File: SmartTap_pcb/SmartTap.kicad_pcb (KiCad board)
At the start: 2 copper layers, 87.1 x 48.9 mm, 18 parts, among them U1 NT3H1101W0FTTJ

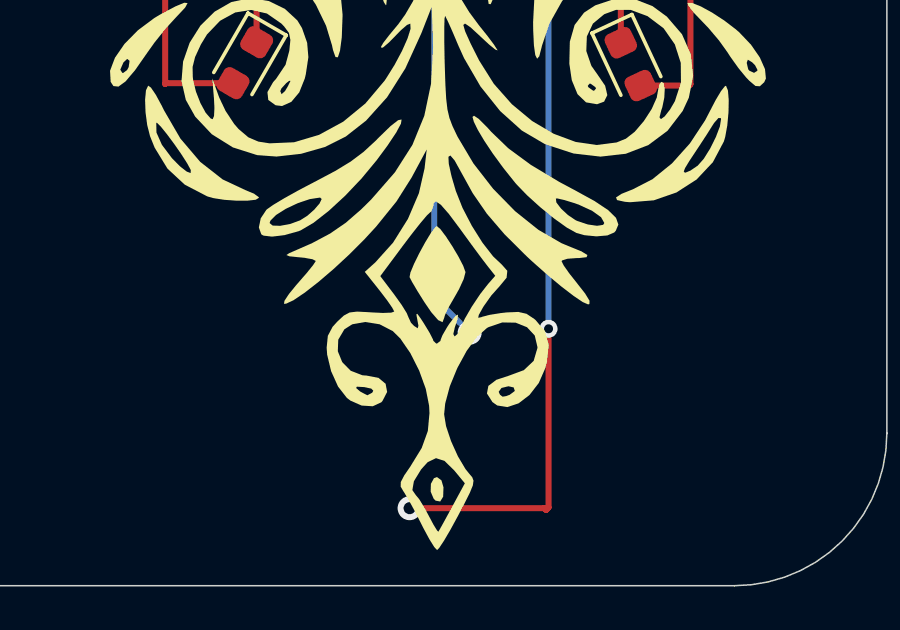
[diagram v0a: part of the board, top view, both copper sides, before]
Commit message: Modified_pcb
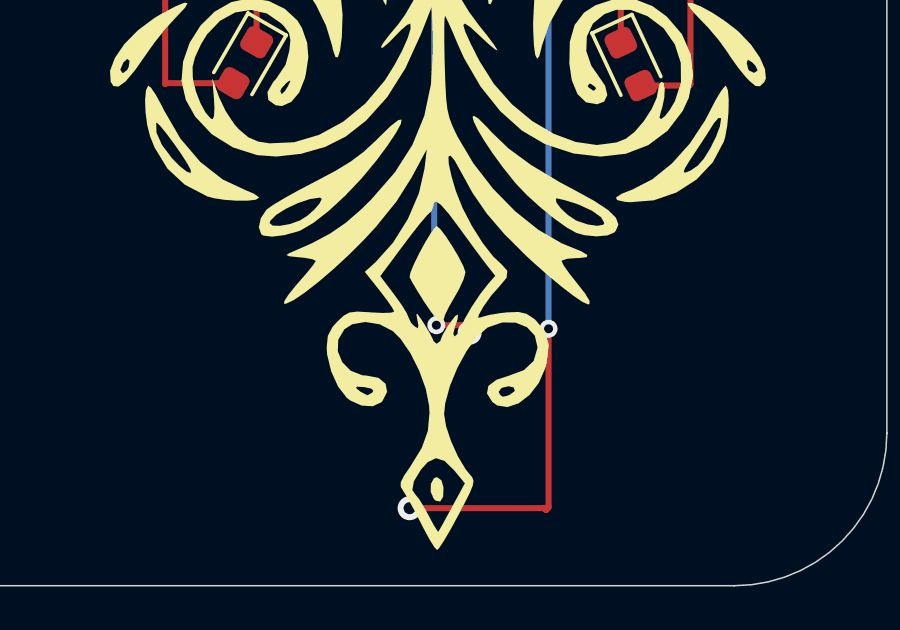
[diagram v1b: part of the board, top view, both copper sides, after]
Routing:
- net lb: track 16.1 -> 17.1 mm, vias 1 -> 2
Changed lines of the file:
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@@
 		(net "la")
+	)
+	(segment
+		(start 178.02 84.03)
+		(end 178.87932 84.03)
+		(width 0.2)
+		(layer "F.Cu")
+		(net "lb")
+	)
+	(segment
+		(start 178.87932 84.03)
+		(end 179.12988 84.28056)
+		(width 0.2)
+		(layer "F.Cu")
+		(net "lb")
+	)
+	(via
+		(at 178.02 84.03)
+		(size 0.6)
+		(drill 0.3)
+		(layers "F.Cu" "B.Cu")
+		(net "lb")
 	)
 	(via
@@
 	(segment
 		(start 177.95 83.10068)
-		(end 178.811781 83.962461)
+		(end 178.02 83.17068)
 		(width 0.2)
 		(layer "B.Cu")
@@
 		(width 0.2)
 		(layer "B.Cu")
+		(net "lb")
+	)
+	(segment
+		(start 178.02 83.17068)
+		(end 178.02 84.03)
+		(width 0.2)
+		(layer "B.Cu")
